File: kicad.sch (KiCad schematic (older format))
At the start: 21 parts, among them J1 Screw_Terminal_01x02, J2 Screw_Terminal_01x03, J3 Screw_Terminal_01x03, J4 Conn_01x05, J5 Screw_Terminal_01x03, SW1 SW_Push, SW2 SW_Push, U6 ESP32

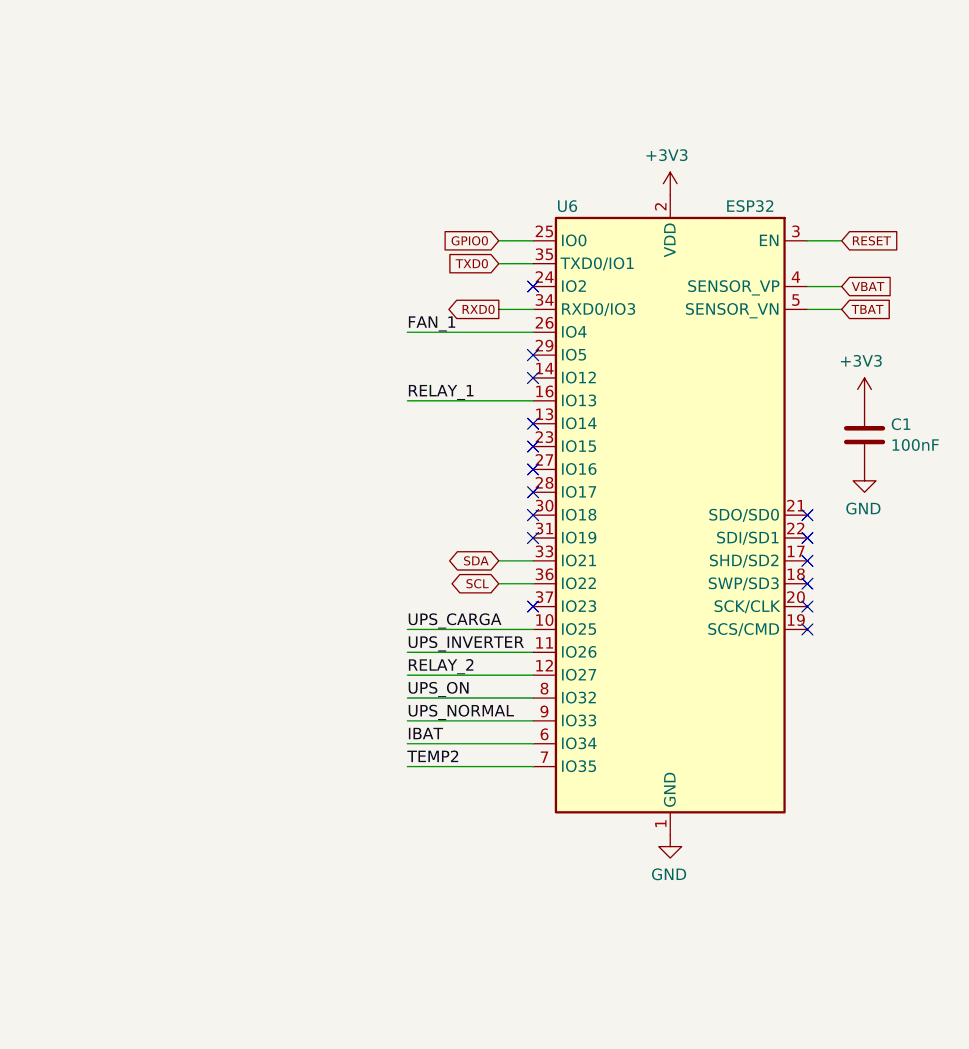
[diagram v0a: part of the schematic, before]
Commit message: various updates
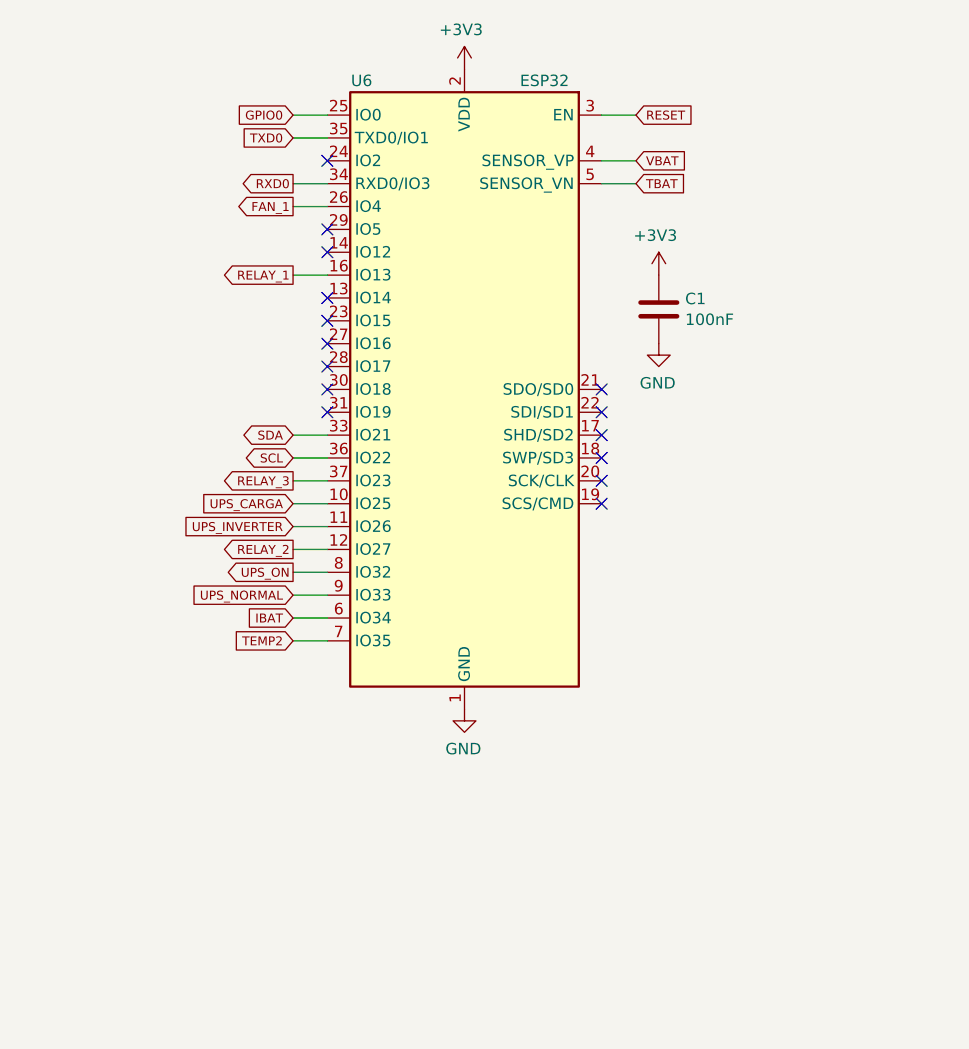
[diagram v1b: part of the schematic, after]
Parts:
- H1, H2: footprint (none) -> MountingHole:MountingHole_4mm_Pad_Via
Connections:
- net RELAY_3: now also U6.37 (IO23)
- no-connect marks 16 -> 15
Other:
- moved on the sheet: C1, U6
